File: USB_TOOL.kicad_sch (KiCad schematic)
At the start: 0 parts

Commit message: update
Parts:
- added U1: ESP32-C3-WROOM-02-N4, ESP32-C3-WROOM-02-N4:ESP32-C3-WROOM-02-N4, symbol ESP32-C3-WROOM-02-N4:ESP32-C3-WROOM-02-N4
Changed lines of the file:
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@@
 	(generator_version "9.0")
 	(paper "A4")
+	(symbol
+		(lib_id "ESP32-C3-WROOM-02-N4:ESP32-C3-WROOM-02-N4")
+		(at 95.25 69.85 0)
+		(unit 1)
+		(exclude_from_sim no)
+		(in_bom yes)
+		(on_board yes)
+		(dnp no)
+		(fields_autoplaced yes)
+		(property "Reference" "U1"
+			(at 95.25 50.8 0)
+			(effects
+				(font
+					(size 1.27 1.27)
+				)
+			)
+		)
+		(property "Value" "ESP32-C3-WROOM-02-N4"
+			(at 95.25 53.34 0)
+			(effects
+				(font
+					(size 1.27 1.27)
+				)
+			)
+		)
+		(property "Footprint" "ESP32-C3-WROOM-02-N4:ESP32-C3-WROOM-02-N4"
+			(at 94.488 94.234 0)
+			(effects
+				(font
+					(size 1.27 1.27)
+				)
+				(hide yes)
+			)
+		)
+		(property "Datasheet" "https://akizukidenshi.com/goodsaffix/esp32-c3-wroom-02_datasheet_en.pdf"
+			(at 86.36 110.49 0)
+			(effects
+				(font
+					(size 1.27 1.27)
+				)
+				(hide yes)
+			)
+		)
+		(property "Description" "ESP32-C3-WROOM-02-N4"
+			(at 92.71 107.188 0)
+			(effects
+				(font
+					(size 1.27 1.27)
+				)
+				(hide yes)
+			)
+		)
+		(property "product" "ESP32-C3-WROOM-02-N4"
+			(at 92.71 107.188 0)
+			(effects
+				(font
+					(size 1.27 1.27)
+				)
+				(hide yes)
+			)
+		)
+		(property "digikey" "none"
+			(at 94.488 94.234 0)
+			(effects
+				(font
+					(size 1.27 1.27)
+				)
+				(hide yes)
+			)
+		)
+		(pin "14"
+		)
+		(pin "7"
+		)
+		(pin "9"
+		)
+		(pin "6"
+		)
+		(pin "16"
+		)
+		(pin "17"
+		)
+		(pin "1"
+		)
+		(pin "19"
+		)
+		(pin "3"
+		)
+		(pin "5"
+		)
+		(pin "8"
+		)
+		(pin "11"
+		)
+		(pin "12"
+		)
+		(pin "4"
+		)
+		(pin "13"
+		)
+		(pin "15"
+		)
+		(pin "18"
+		)
+		(pin "2"
+		)
+		(pin "10"
+		)
+		(instances
+			(project ""
+				(path "/232069e4-b86e-45a3-b9aa-f0b54358ce0d"
+					(reference "U1")
+					(unit 1)
+				)
+			)
+		)
+	)
 	(sheet_instances
 		(path "/"

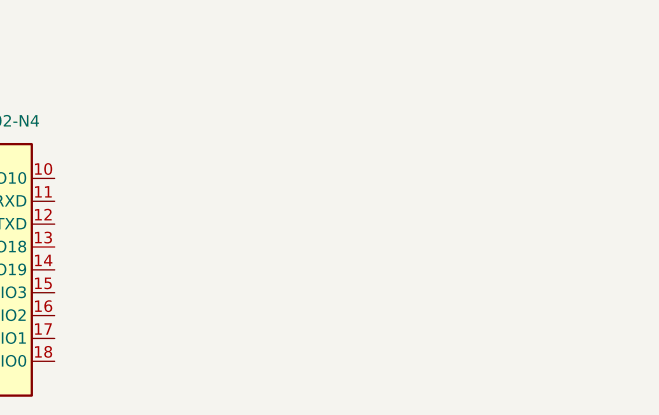
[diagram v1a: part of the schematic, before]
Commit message: pull
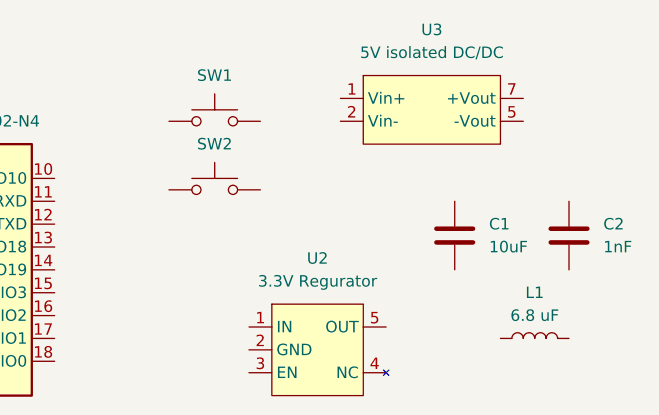
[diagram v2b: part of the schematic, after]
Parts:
- added C1: 10uF, Capacitor_SMD:C_1206_3216Metric, symbol CL31B106KAHNNNE:CL31B106KAHNNNE
- added C2: 1nF, Capacitor_SMD:C_1808_4520Metric, symbol C1808X102K402T:C1808X102K402T
- added L1: 6.8 uF, Inductor_SMD:L_1210_3225Metric, symbol WIP322512A-6R8MLDG:WIP322512A-6R8MLDG
- added SW1, SW2: ~, Button_Switch_THT:SW_PUSH_1P1T_6x3.5mm_H4.3_APEM_MJTP1243, symbol GSPTS003907:GSPTS003907
- added U2: 3.3V Regurator, Package_TO_SOT_SMD:SOT-23-5, symbol AP7366EA-33W5-7:AP7366EA-33W5-7
- added U3: 5V isolated DC/DC, AM3DS-0505SH30LPZ:AM3DS-0505SH30LPZ, symbol AM3DS-0505SH30LPZ:AM3DS-0505SH30LPZ

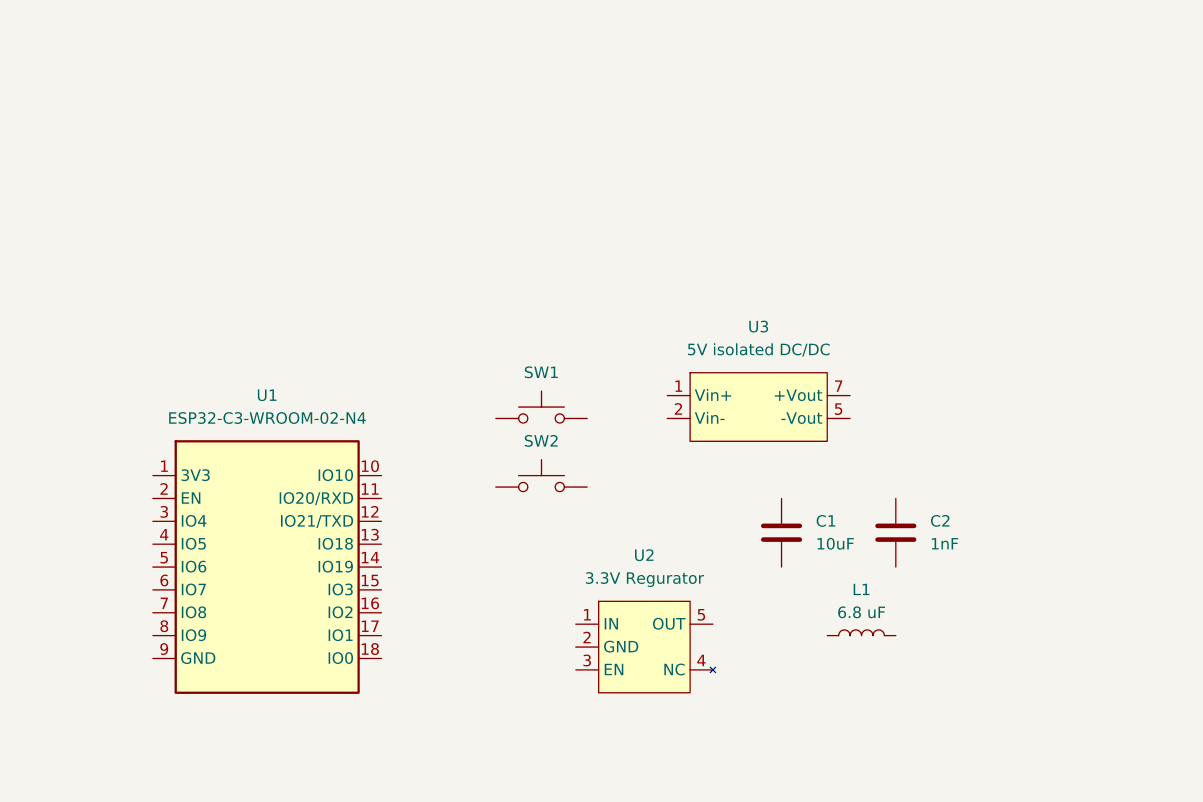
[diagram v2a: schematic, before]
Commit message: uo
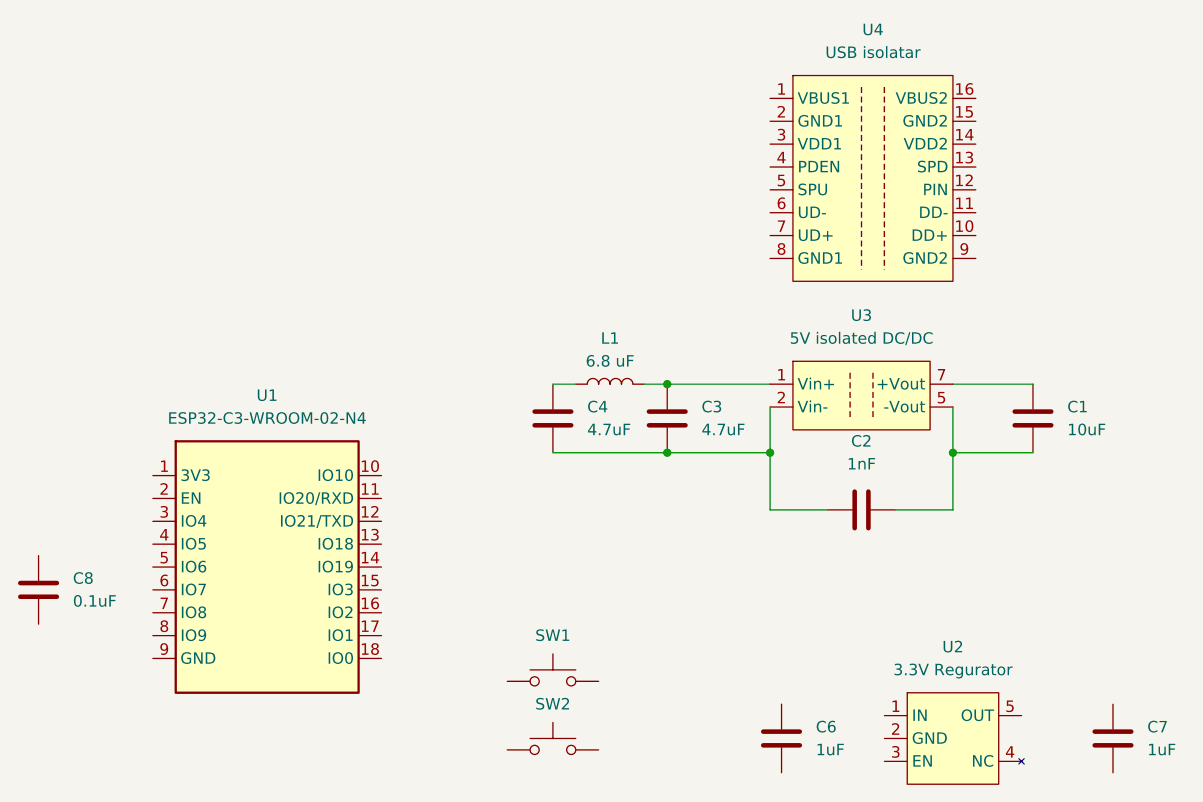
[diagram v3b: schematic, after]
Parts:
- added C3, C4: 4.7uF, Capacitor_SMD:C_0603_1608Metric, symbol GRM188R61E475KE11D:GRM188R61E475KE11D
- added C6, C7: 1uF, Capacitor_SMD:C_0805_2012Metric, symbol CL21B105KBFNNNE:CL21B105KBFNNNE
- added C8: 0.1uF, Capacitor_SMD:C_0603_1608Metric, symbol GRM188F11H104ZA01:GRM188F11H104ZA01
- added U4: USB isolatar, Package_SO:SOIC-16W_7.5x10.3mm_P1.27mm, symbol ADUM3160BRWZ-RL:ADUM3160BRWZ-RL
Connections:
- net at U3.1 (Vin+): now also L1.2, C3.1
- net at U3.2 (Vin-): now also C2.1, C3.2, C4.2
- net at U3.5 (-Vout): now also C1.2, C2.2
- net at U3.7 (+Vout): now also C1.1
- net at L1.1: now also C4.1
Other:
- moved on the sheet: C1, C2, L1, SW1, SW2, U2

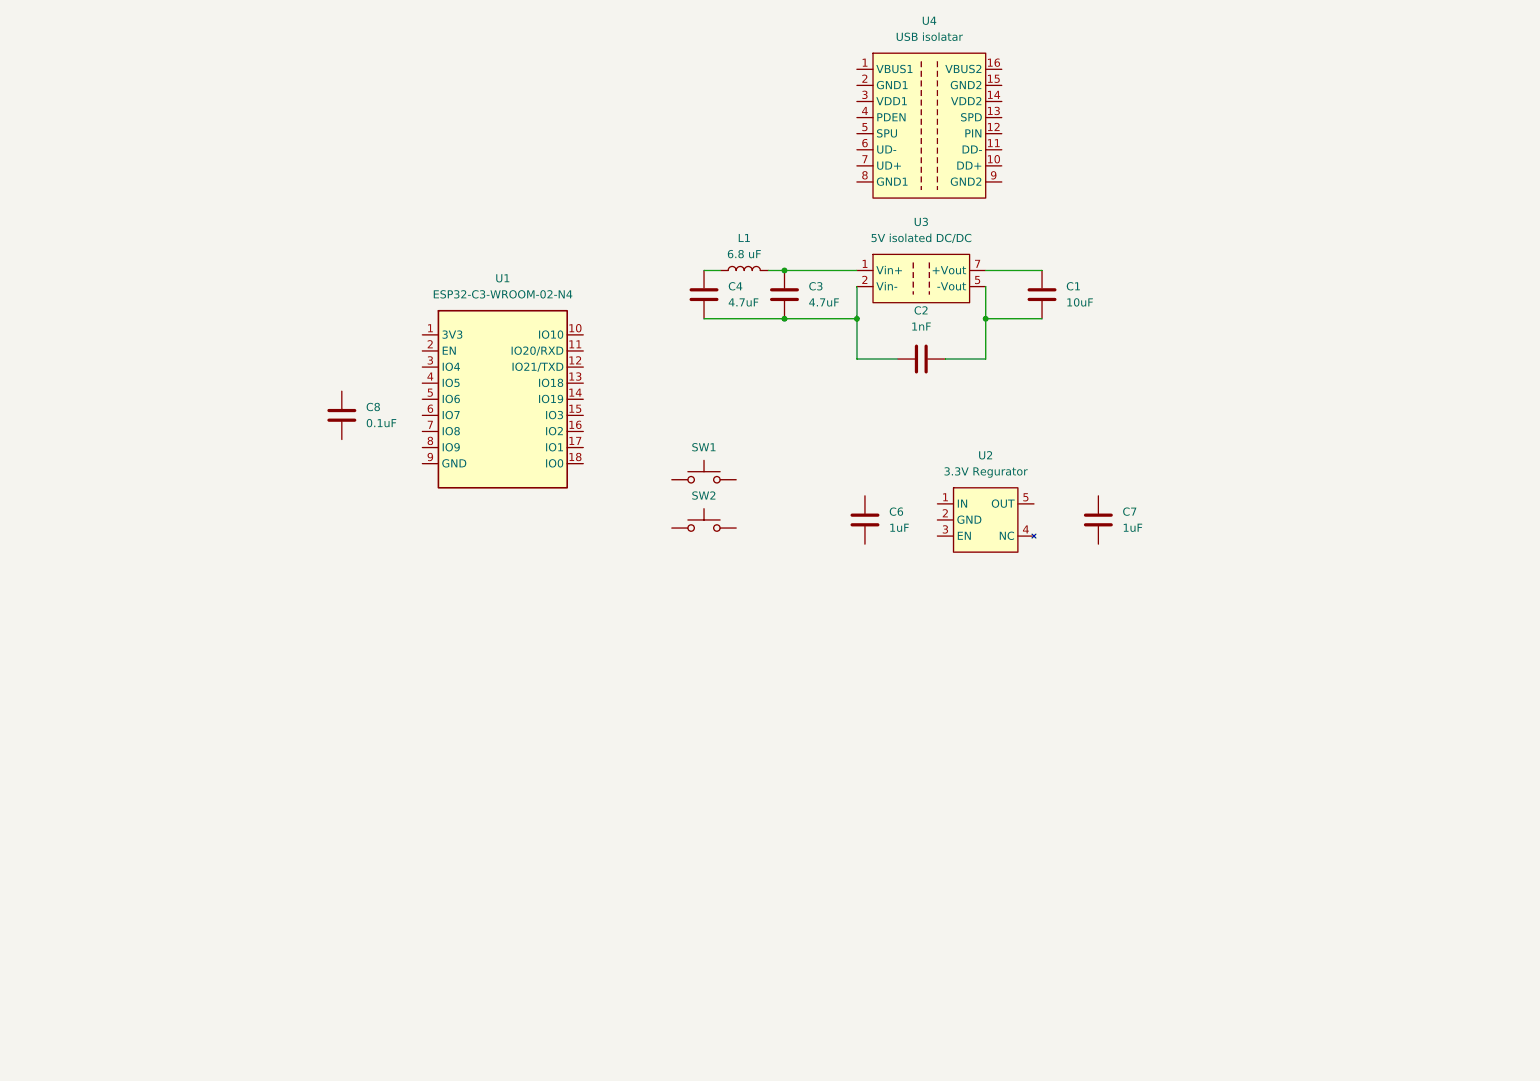
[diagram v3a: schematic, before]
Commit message: asd
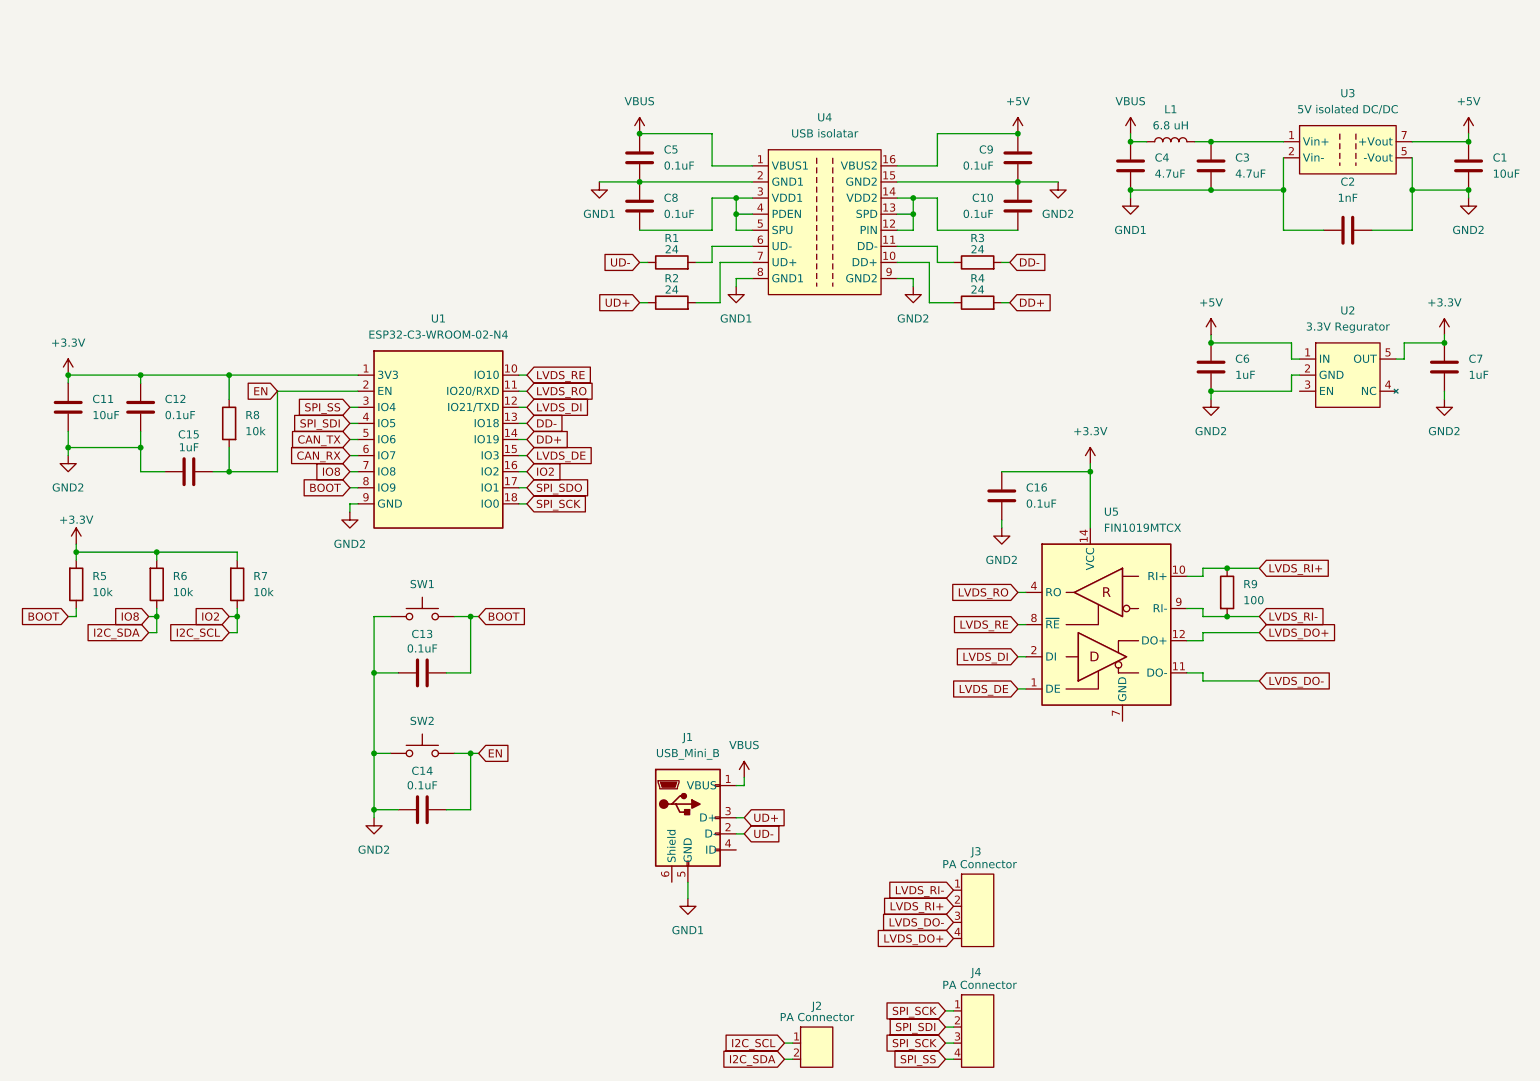
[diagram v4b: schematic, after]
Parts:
- added C10, C12, C13, C14, C16, C5, C9: 0.1uF, Capacitor_SMD:C_0603_1608Metric, symbol GRM188F11H104ZA01:GRM188F11H104ZA01
- added C11: 10uF, Capacitor_SMD:C_1206_3216Metric, symbol CL31B106KAHNNNE:CL31B106KAHNNNE
- added C15: 1uF, Capacitor_SMD:C_0805_2012Metric, symbol CL21B105KBFNNNE:CL21B105KBFNNNE
- added J1: USB_Mini_B, MUSB-5BF01AS:MUSB-5BF01AS, symbol MUSB-5BF01AS:MUSB-5BF01AS
- added J2: PA Connector, S02B-PASK-2:S02B-PASK-2, symbol S02B-PASK-2:S02B-PASK-2
- added J3, J4: PA Connector, S04B-PASK-2:S04B-PASK-2, symbol S04B-PASK-2:S04B-PASK-2
- added R1, R2, R3, R4: 24, Resistor_SMD:R_0402_1005Metric, symbol RC0402FR-0724RL:RC0402FR-0724RL
- added R5, R6, R7, R8: 10k, Resistor_SMD:R_0603_1608Metric, symbol NRC06F1002TRF:NRC06F1002TRF
- added R9: 100, Resistor_SMD:R_0402_1005Metric, symbol RK73H1ETTP1000F:RK73H1ETTP1000F
- added U5: FIN1019MTCX, Package_SO:TSSOP-14_4.4x5mm_P0.65mm, symbol FIN1019MTCX:FIN1019MTCX
- L1: value 6.8 uF -> 6.8 uH
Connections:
- net +3.3V: now reaches U1.1 (3V3)
- net +3.3V: now also C7.1, U2.5 (OUT), C11.1, C12.1, C16.1, R5.1, R6.1, R7.1, R8.2, U5.14 (VCC)
- net LVDS_RE: now reaches U1.10 (IO10)
- net LVDS_RE: now also U5.8 (~{RE})
- net LVDS_RO: now reaches U1.11 (IO20/RXD)
- net LVDS_RO: now also U5.4 (RO)
- net LVDS_DI: now reaches U1.12 (IO21/TXD)
- net LVDS_DI: now also U5.2 (DI)
- net DD-: now reaches U1.13 (IO18)
- net DD-: now also R3.2
- net DD+: now reaches U1.14 (IO19)
- net DD+: now also R4.2
- net LVDS_DE: now reaches U1.15 (IO3)
- net LVDS_DE: now also U5.1 (DE)
- net I2C_SCL: now reaches U1.16 (IO2)
- net I2C_SCL: now also J2.1, R7.2
- net SPI_SDO: now reaches U1.17 (IO1)
- net SPI_SCK: now reaches U1.18 (IO0)
- net SPI_SCK: now also J4.1, J4.3
- net EN: now reaches U1.2 (EN)
- net EN: now also SW2.2, C14.2, C15.2, R8.1
- net SPI_SS: now reaches U1.3 (IO4)
- net SPI_SS: now also J4.4
- net SPI_SDI: now reaches U1.4 (IO5)
- net SPI_SDI: now also J4.2
- net CAN_TX: now reaches U1.5 (IO6)
- net CAN_RX: now reaches U1.6 (IO7)
- net I2C_SDA: now reaches U1.7 (IO8)
- net I2C_SDA: now also J2.2, R6.2
- net BOOT: now reaches U1.8 (IO9)
- net BOOT: now also SW1.2, C13.2, R5.2
- net GND2: now reaches U1.9 (GND)
- net GND2: now also C1.2, C2.2, C6.2, C7.2, SW1.1, SW2.1, U2.2 (GND), U3.5 (-Vout), U4.15 (GND2), U4.9 (GND2), C10.1, C11.2, C12.2, C13.1, C14.1, C15.1, C16.2, C9.2
- net GND1: now reaches C2.1, C3.2, C4.2, U3.2 (Vin-)
- net GND1: now also C8.1, U4.2 (GND1), U4.8 (GND1), C5.2, J1.5 (GND)
- net +5V: now reaches C1.1, U3.7 (+Vout)
- net +5V: now also C6.1, U2.1 (IN), U4.16 (VBUS2), C9.1
- net at C8.2: now also U4.3 (VDD1), U4.4 (PDEN), U4.5 (SPU)
- net VBUS: now reaches C4.1, L1.1
- net VBUS: now also U4.1 (VBUS1), C5.1, J1.1 (VBUS)
- net at U4.10 (DD+): now also R4.1
- net at U4.11 (DD-): now also R3.1
- net at U4.12 (PIN): now also U4.13 (SPD), U4.14 (VDD2), C10.2
- net at U4.6 (UD-): now also R1.2
- net at U4.7 (UD+): now also R2.2
- new net LVDS_DO+: J3.4, U5.12 (DO+)
- new net LVDS_DO-: J3.3, U5.11 (DO-)
- new net LVDS_RI+: J3.2, R9.1, U5.10 (RI+)
- new net LVDS_RI-: J3.1, R9.2, U5.9 (RI-)
- new net UD+: J1.3 (D+), R2.1
- new net UD-: J1.2 (D-), R1.1
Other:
- moved on the sheet: C1, C2, C3, C4, C6, C7, C8, L1, SW1, SW2, U1, U2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
